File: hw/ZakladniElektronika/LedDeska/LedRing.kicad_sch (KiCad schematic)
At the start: 120 parts

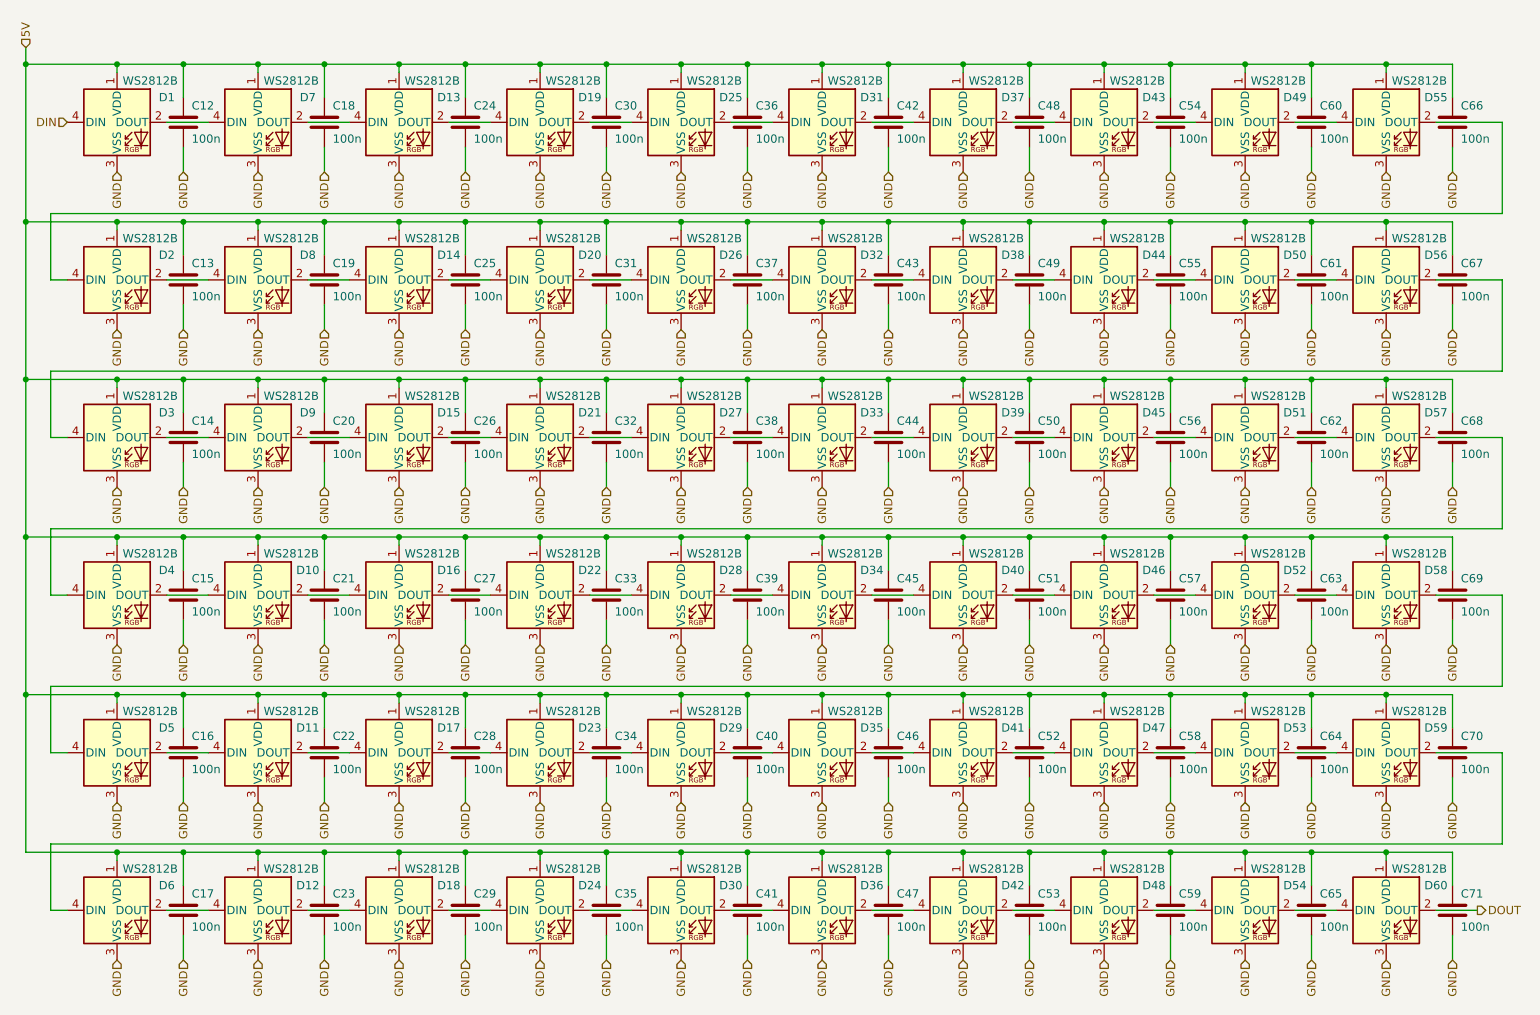
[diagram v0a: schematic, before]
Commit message: WIP
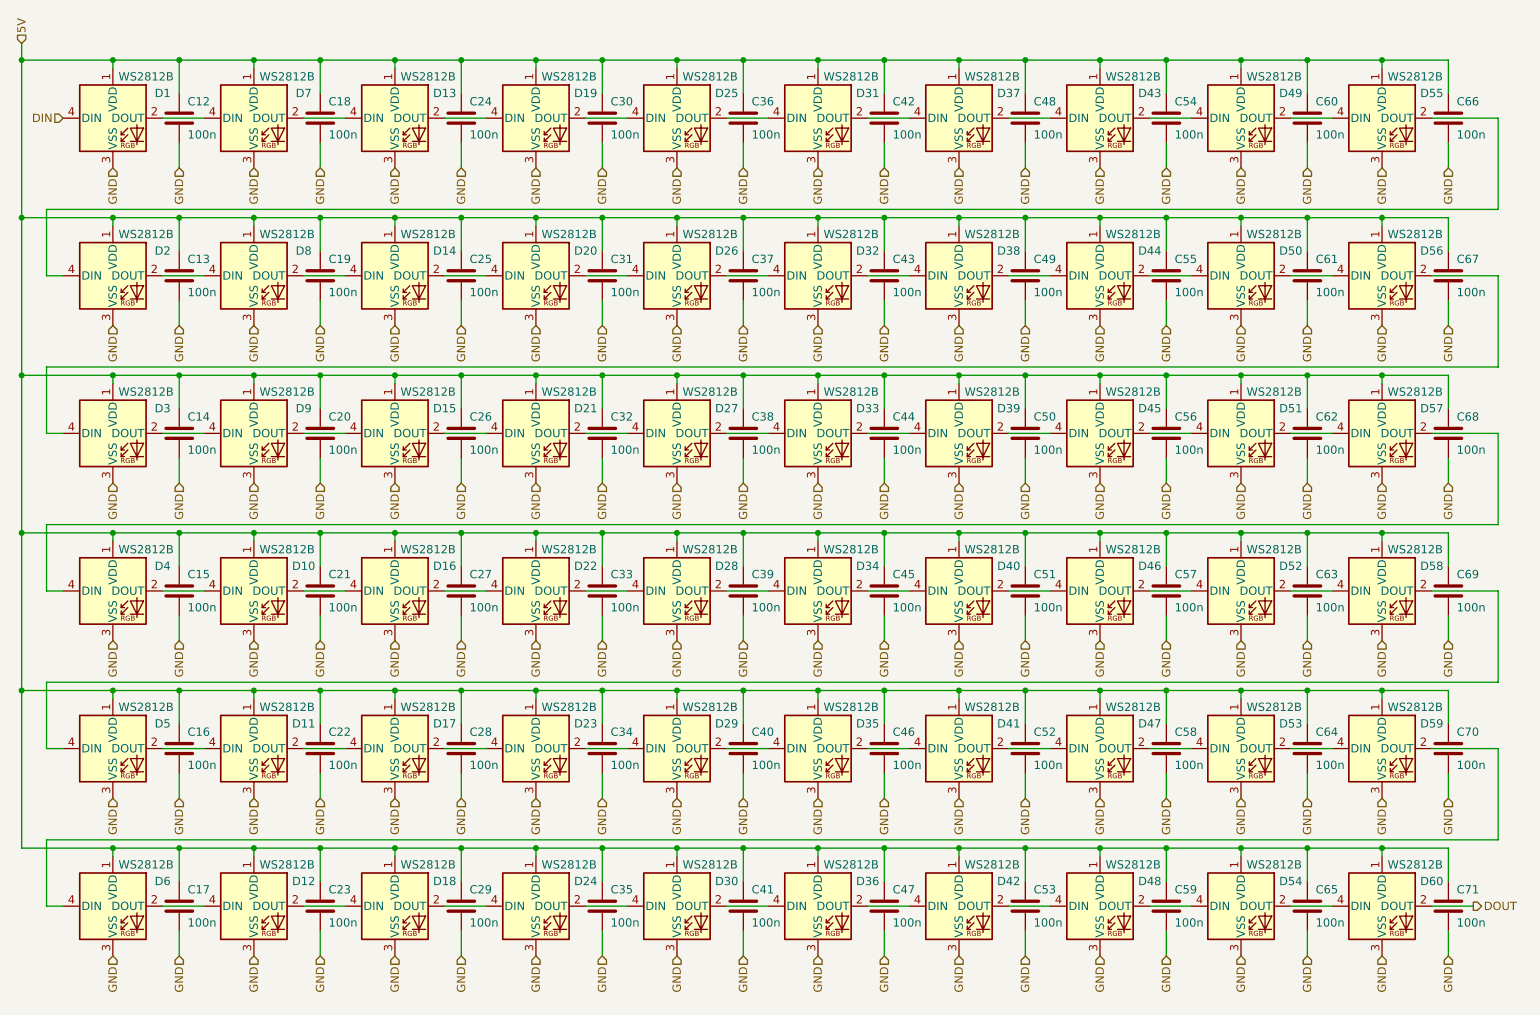
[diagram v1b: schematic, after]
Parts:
- C12, C13, C14, C15, C16, C17, C18, C19, C20, C21, C22, C23, C24, C25, C26, C27, C28, C29, C30, C31, C32, C33, C34, C35, C36, C37, C38, C39, C40, C41, C42, C43, C44, C45, C46, C47, C48, C49, C50, C51, C52, C53, C54, C55, C56, C57, C58, C59, C60, C61, C62, C63, C64, C65, C66, C67, C68, C69, C70, C71: Basic/Extended (none) -> B; LCSC (none) -> C307331; info (none) -> 50V, X7R
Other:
- moved on the sheet: C12, C13, C14, C15, C16, C17, C18, C19, C20, C21, C22, C23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

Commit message: Likvidace MiniUI jako samostatné desky a výběr všech komponent
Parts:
- D1, D10, D11, D12, D13, D14, D15, D16, D17, D18, D19, D2, D20, D21, D22, D23, D24, D25, D26, D27, D28, D29, D3, D30, D31, D32, D33, D34, D35, D36, D37, D38, D39, D4, D40, D41, D42, D43, D44, D45, D46, D47, D48, D49, D5, D50, D51, D52, D53, D54, D55, D56, D57, D58, D59, D6, D60, D7, D8, D9: footprint RB3203-Lib:WS2812 -> RKL-LED:3528RGBW-WS2812B; Basic/Extended (none) -> E; LCSC (none) -> C2890364
